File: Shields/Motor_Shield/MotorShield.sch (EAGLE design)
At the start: 38 parts, among them U1 ATMEGA328P_TQFP, U3 FT232RL, X1 2510-, X2 2510-, X3 C-GRID-05-15-91, X4 C-GRID-05-15-91, X5 MINI-USB_4P-32005-101, Y1 16MHz

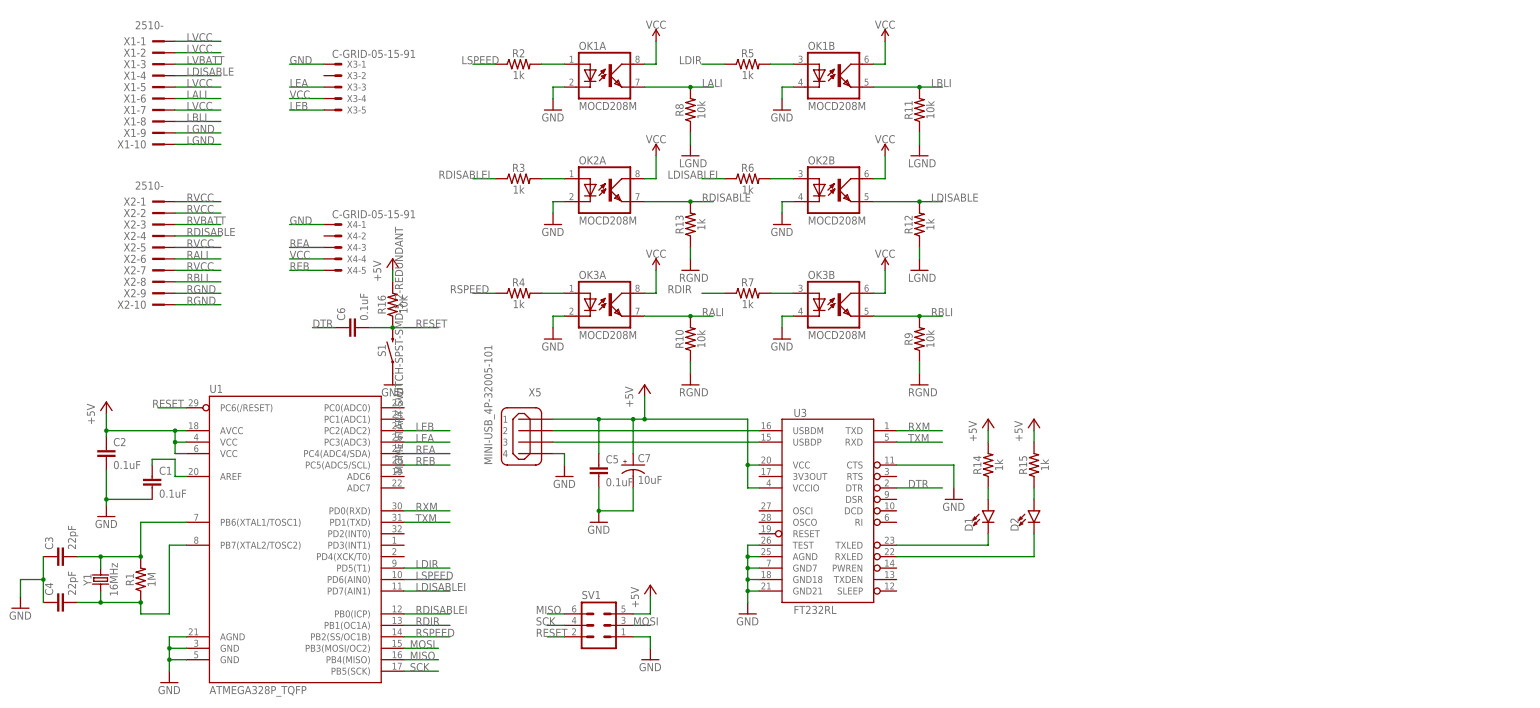
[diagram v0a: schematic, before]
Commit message: motor and light board
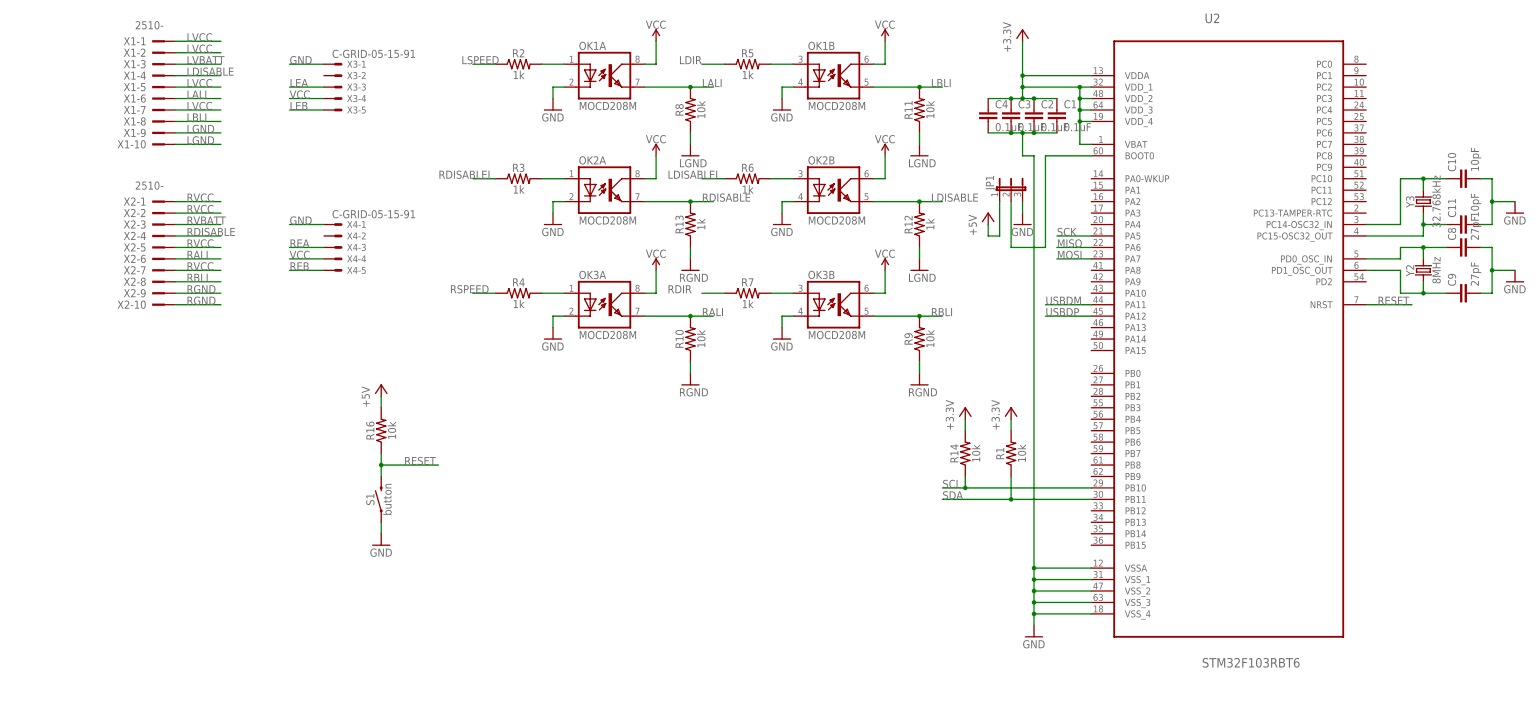
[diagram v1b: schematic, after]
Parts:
- removed C5, C6: 0.1uF, SparkFun-Capacitors:0.1UF-0603-25V-(+80/-20%)
- removed C7: 10uF, SparkFun-Capacitors:10UF-POLAR-0603-6.3V-20%(TANT)
- removed D1, D2: (no value), SparkFun-LED:LED0603
- removed R15: 1k, SparkFun-Resistors:1KOHM-0603-1/10W-1%
- removed SV1: (no value), con-lstb:MA03-2
- removed U1: ATMEGA328P_TQFP, SparkFun-IC-Microcontroller:ATMEGA328P_TQFP
- removed U3: FT232RL, SparkFun-IC-Comms:FT232RLSSOP
- removed X5: MINI-USB_4P-32005-101, con-cypressindustries:MINI-USB_4P-32005-101
- removed Y1: 16MHz, SparkFun-Clocks:CRYSTAL-16MHZPTH-HC49US
- added C10, C11: 10pF, SparkFun-Capacitors:10PF-0603-50V-5%
- added C8, C9: 27pF, SparkFun-Capacitors:27PF-0603-50V-5%
- added JP1: (no value), jumper:JP2E
- added U2: STM32F103RBT6, ST Microelctronics_By_element14_Batch_1:STM32F103RBT6
- added Y2: 8MHz, SparkFun-Clocks:CRYSTAL-8MHZSMD-5X3.2
- added Y3: 32.768kHz, SparkFun-Clocks:CRYSTAL-32.768KHZSMD-3.2X1.5
- C3, C4: value 22pF -> 0.1uF; device SparkFun-Capacitors:22PF-0603-50V-5% -> SparkFun-Capacitors:0.1UF-0603-25V-(+80/-20%)
- R1: value 1M -> 10k; device SparkFun-Resistors:1MOHM-0603-1/4W-5% -> SparkFun-Resistors:10KOHM-0603-1/10W-1%
- R14: value 1k -> 10k; device SparkFun-Resistors:1KOHM-0603-1/10W-1% -> SparkFun-Resistors:10KOHM-0603-1/10W-1%
- S1: value MOMENTARY-SWITCH-SPST-SMD-5.2-REDUNDANT -> button
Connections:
- removed net DTR: C6.1, U3.DTR
- removed net N$10: U3.USBDM, X5.2
- removed net N$11: U3.USBDP, X5.3
- removed net N$14: D1.A, R14.1
- removed net N$15: D2.A, R15.1
- removed net N$16: D1.C, U3.TXLED
- removed net N$17: D2.C, U3.RXLED
- removed net N$3: C3.2, R1.2, U1.PB6(XTAL1/TOSC1), Y1.2
- removed net N$4: C4.2, R1.1, U1.PB7(XTAL2/TOSC2), Y1.1
- removed net RXM: U1.PD0(RXD), U3.TXD
- removed net TXM: U1.PD1(TXD), U3.RXD
- new net +3.3V: C1.1, C2.1, C3.1, C4.1, U2.VBAT, U2.VDDA, U2.VDD_1, U2.VDD_2, U2.VDD_3, U2.VDD_4
- new net +5V: JP1.1, R1.2, R14.2
- new net N$12: C8.1, U2.PD0_OSC_IN, Y2.2
- new net N$13: C9.1, U2.PD1_OSC_OUT, Y2.1
- new net N$19: C11.1, U2.PC15-OSC32_OUT, Y3.1
- new net N$20: C10.1, U2.PC14-OSC32_IN, Y3.2
- new net SCL: R14.1, U2.PB10
- new net SDA: R1.1, U2.PB11
- new net USBDM: U2.PA11
- new net USBDP: U2.PA12
- net GND: now also C10.2, C11.2, C3.2, C4.2, C8.2, C9.2, JP1.3, U2.VSSA, U2.VSS_1, U2.VSS_2, U2.VSS_3, U2.VSS_4; no longer C3.1, C4.1, C5.2, C7.-, SV1.1, U1.AGND, U1.GND@3, U1.GND@5, U3.AGND, U3.CTS, U3.GND18, U3.GND21, U3.GND7, U3.TEST, X5.4
- net LDIR: no longer U1.PD5(T1)
- net LDISABLEI: no longer U1.PD7(AIN1)
- net LEA: no longer U1.PC3(ADC3)
- net LEB: no longer U1.PC2(ADC2)
- net LSPEED: no longer U1.PD6(AIN0)
- net MISO: now also U2.PA6; no longer SV1.6, U1.PB4(MISO)
- net MOSI: now also U2.PA7; no longer SV1.3, U1.PB3(MOSI/OC2)
- net N$2: now also JP1.2, U2.BOOT0; no longer C1.1, U1.AREF
- net RDIR: no longer U1.PB1(OC1A)
- net RDISABLEI: no longer U1.PB0(ICP)
- net REA: no longer U1.PC4(ADC4/SDA)
- net REB: no longer U1.PC5(ADC5/SCL)
- net RESET: now also U2.NRST; no longer C6.2, SV1.2, U1.PC6(/RESET)
- net RSPEED: no longer U1.PB2(SS/OC1B)
- net SCK: now also U2.PA5; no longer SV1.4, U1.PB5(SCK)
- net VCC: no longer C2.1, C5.1, C7.+, R14.2, R15.2, SV1.5, U1.AVCC, U1.VCC@4, U1.VCC@6, U3.VCC, U3.VCCIO, X5.1
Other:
- moved on the sheet: C1, C2, C3, C4, R1, R14, R16, S1
